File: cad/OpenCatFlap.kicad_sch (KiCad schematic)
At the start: 17 parts, among them P1 Outside PIR, P2 IR Barrier Outside, P3 IR Barrier Inside, P4 Servo Outside, P5 Servo Inside, P6 RFID inside, P7 RFID outside, U1 DOIT-ESP32-DEVKIT-V1, U2 AMN33111, U3 5V

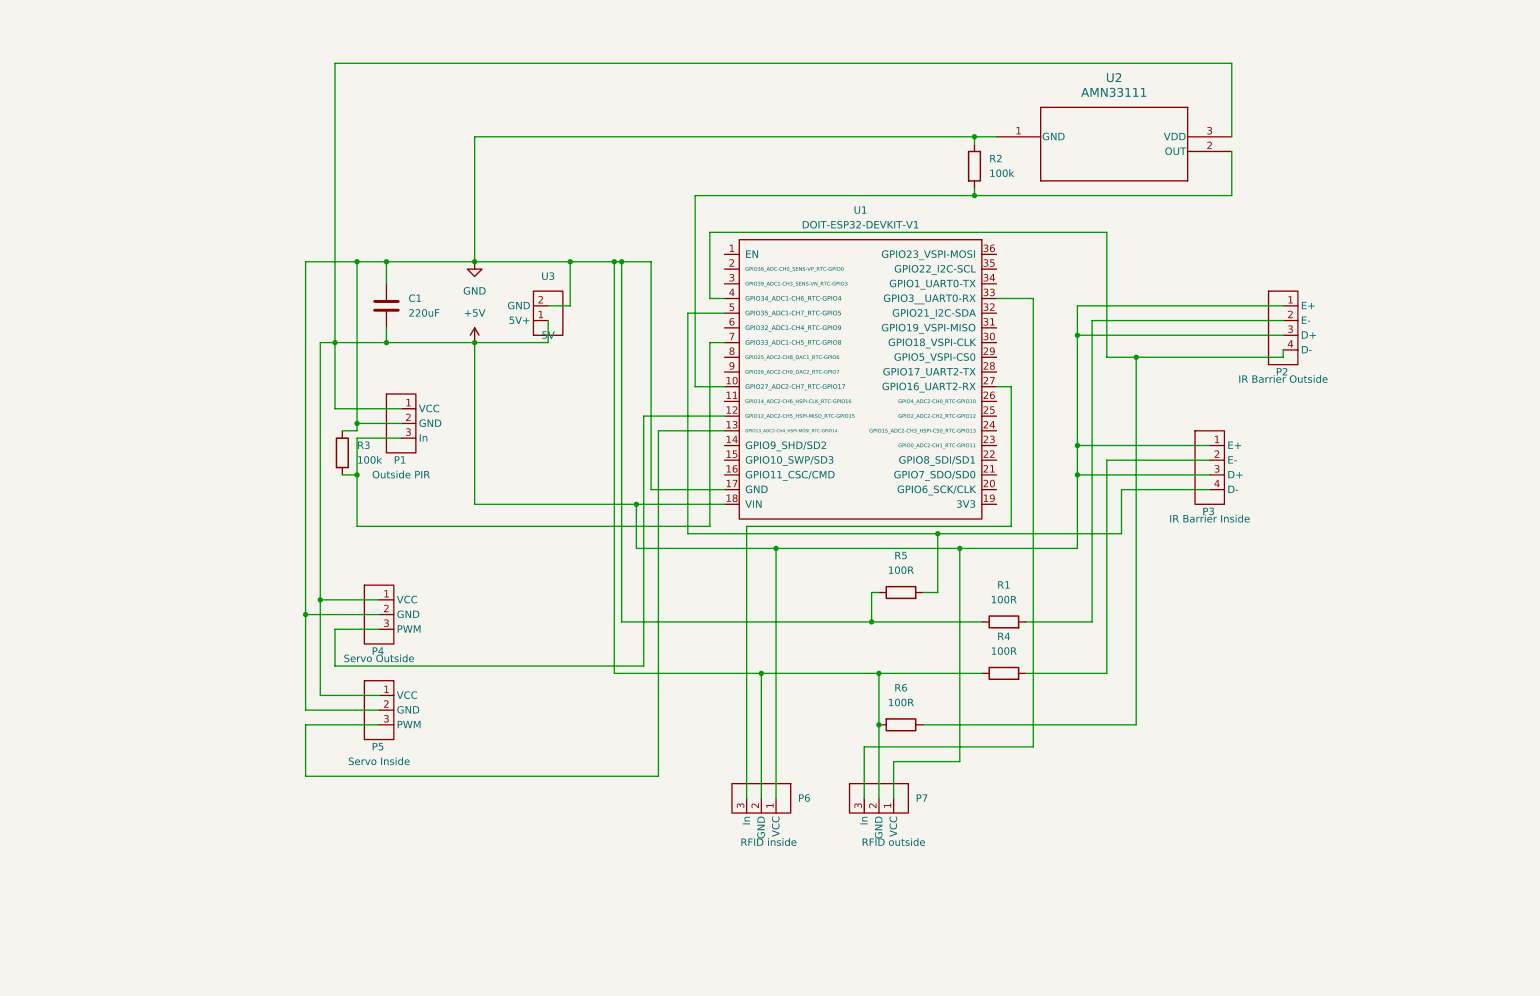
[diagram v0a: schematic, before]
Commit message: meow
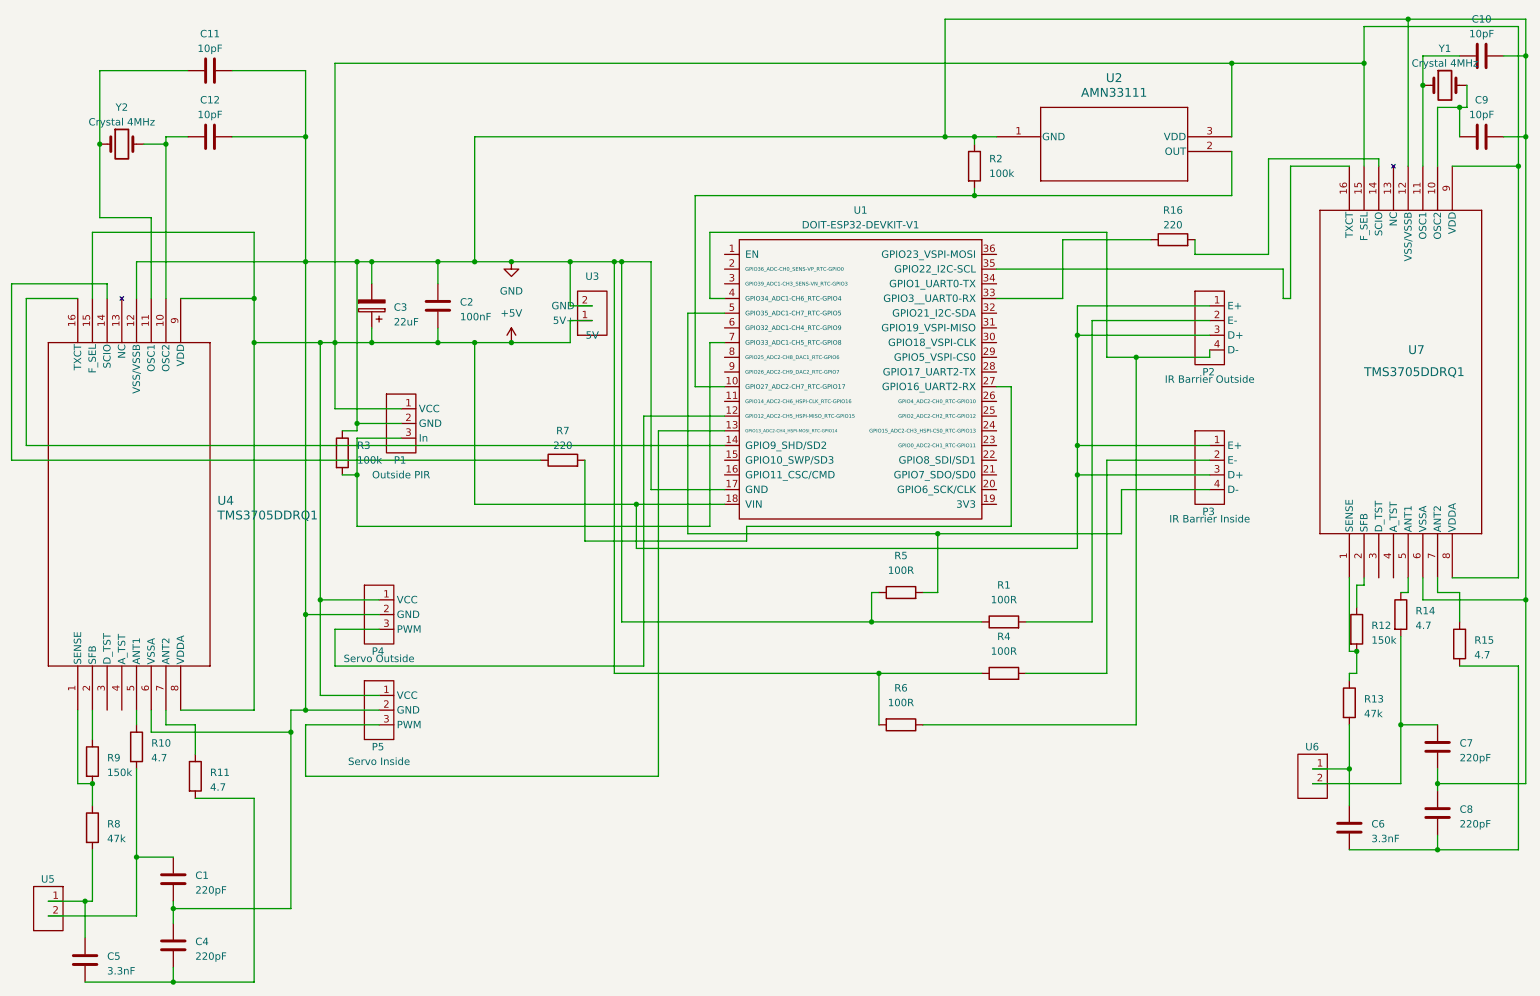
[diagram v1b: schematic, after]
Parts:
- removed P6: RFID inside, OpenCatFlap:PIR Header, symbol OpenCatFlap:PIR Header
- removed P7: RFID outside, OpenCatFlap:PIR Header, symbol OpenCatFlap:PIR Header
- added C10, C11, C12, C9: 10pF, Capacitor_SMD:C_0805_2012Metric, symbol Device:C
- added C2: 100nF, Capacitor_SMD:C_0805_2012Metric, symbol Device:C
- added C3: 22uF, Capacitor_SMD:CP_Elec_8x10, symbol Device:C_Polarized
- added C4, C7, C8: 220pF, Capacitor_SMD:C_0805_2012Metric, symbol Device:C
- added C5, C6: 3.3nF, Capacitor_SMD:C_0805_2012Metric, symbol Device:C
- added R10, R11, R14, R15: 4.7, Resistor_SMD:R_0805_2012Metric, symbol Device:R
- added R12, R9: 150k, Resistor_SMD:R_0805_2012Metric, symbol Device:R
- added R13, R8: 47k, Resistor_SMD:R_0805_2012Metric, symbol Device:R
- added R16, R7: 220, Resistor_SMD:R_0805_2012Metric, symbol Device:R
- added U4, U7: TMS3705DDRQ1, D16, symbol OpenCatFlap:TMS3705DDRQ1
- added U5, U6: ~, OpenCatFlap:Power Header, symbol OpenCatFlap:Power_Plug
- added Y1, Y2: Crystal 4MHz, Crystal:Crystal_HC49-4H_Vertical, symbol Device:Crystal
- C1: value 220uF -> 220pF; footprint Capacitor_THT:CP_Radial_D5.0mm_P2.50mm -> Capacitor_SMD:C_0805_2012Metric
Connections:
- net +5V: now also C2.2, C3.1, U4.15 (F_SEL), U4.8 (VDDA), U4.9 (VDD), U7.15 (F_SEL), U7.8 (VDDA), U7.9 (VDD); no longer C1.2
- net GND: now also C1.2, C10.2, C11.2, C12.2, C2.1, C3.2, C4.1, C7.2, C8.1, C9.2, U4.12 (VSS/VSSB), U4.6 (VSSA), U7.12 (VSS/VSSB), U7.6 (VSSA); no longer C1.1
- net at U1.33 (GPIO3__UART0-RX): now also R16.1
- net at U1.27 (GPIO16_UART2-RX): now also R7.2
- net at U1.14 (GPIO9_SHD/SD2): now also U4.16 (TXCT)
- net at U1.35 (GPIO22_I2C-SCL): now also U7.16 (TXCT)
- new net: C6.1, R13.2, U6.1 (5V+)
- new net: C6.2, C8.2, R15.2
- new net: C12.1, U4.10 (OSC2), Y2.2
- new net: C10.1, U7.11 (OSC1), Y1.1
- new net: C1.1, R10.2, U5.2 (GND)
- new net: C5.1, R8.2, U5.1 (5V+)
- new net: C4.2, C5.2, R11.2
- new net: R8.1, R9.2, U4.1 (SENSE)
- new net: C11.1, U4.11 (OSC1), Y2.1
- new net: R7.1, U4.14 (SCIO)
- new net: R9.1, U4.2 (SFB)
- new net: R10.1, U4.5 (ANT1)
- new net: R11.1, U4.7 (ANT2)
- new net: C9.1, U7.10 (OSC2), Y1.2
- new net: R12.1, U7.2 (SFB)
- new net: R12.2, R13.1, U7.1 (SENSE)
- new net: R16.2, U7.14 (SCIO)
- new net: R14.1, U7.5 (ANT1)
- new net: R15.1, U7.7 (ANT2)
- new net: C7.1, R14.2, U6.2 (GND)
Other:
- moved on the sheet: P2, U3
